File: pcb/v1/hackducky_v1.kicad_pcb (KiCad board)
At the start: 2 copper layers, 70 x 19 mm, 45 parts, among them J1 USB_C_Receptacle_USB2.0_16P, J2 Micro_SD_Card, J3 USB_A, SW1 SW_Push, SW2 SW_Push, U1 XC6206PxxxMR, U2 W25Q64JVZPIQ, U3 RP2040, Y1 Crystal_GND23

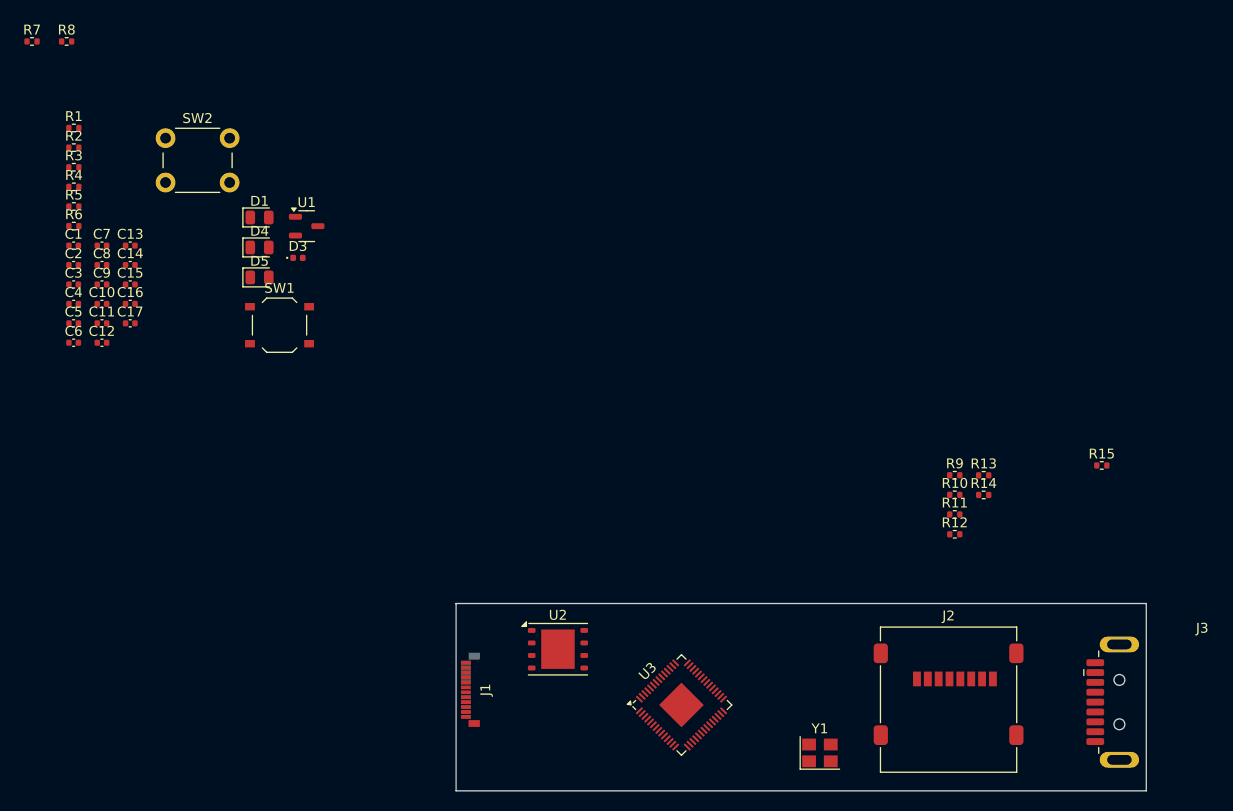
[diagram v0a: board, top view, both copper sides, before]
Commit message: edit stuff
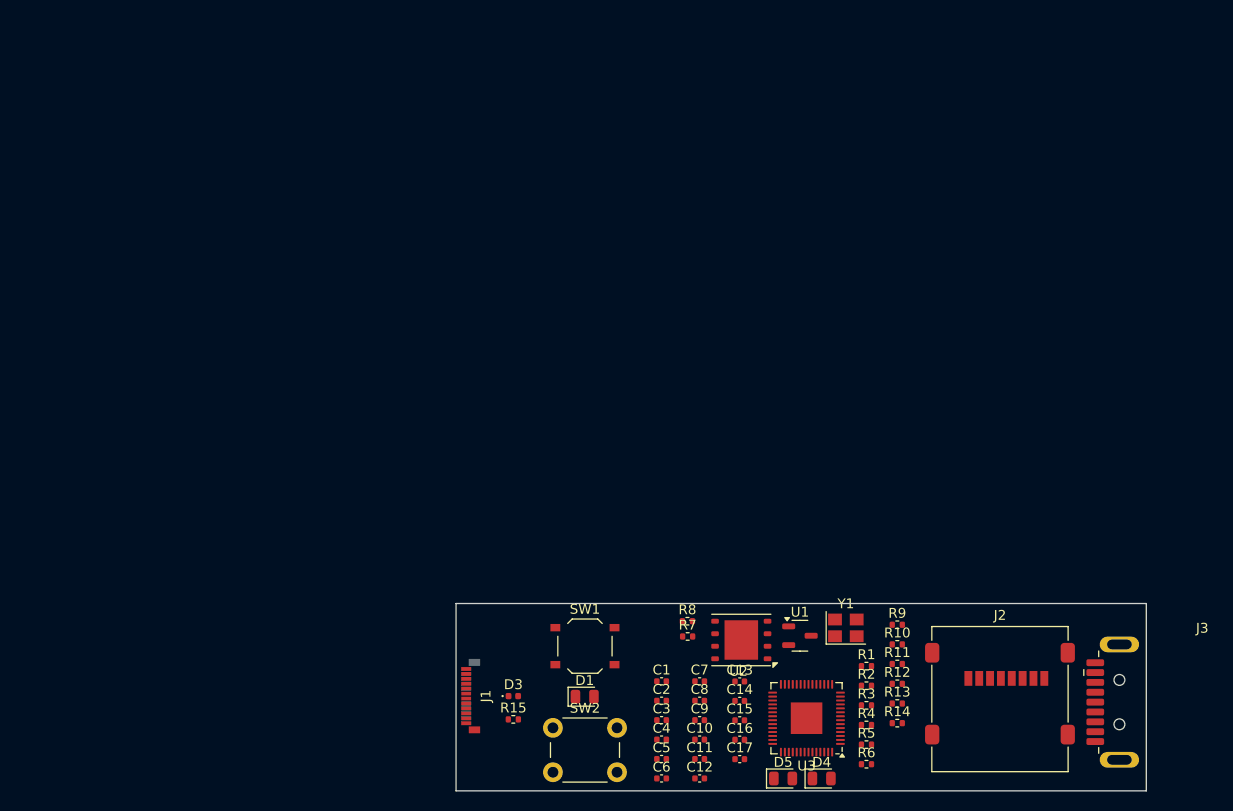
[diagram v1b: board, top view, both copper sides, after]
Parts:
- moved R1 97.2 mm to (120.6, 88.3)
- moved R2 97.2 mm to (120.6, 90.3)
- moved R3 97.2 mm to (120.6, 92.3)
- moved R4 97.2 mm to (120.6, 94.3)
- moved R5 97.2 mm to (120.6, 96.3)
- moved R6 97.2 mm to (120.6, 98.3)
- moved R7 89.8 mm to (102.5, 85.3)
- moved R8 86.1 mm to (102.5, 83.8)
- moved D4 78.4 mm to (116.1, 99.7)
- moved C15 76.0 mm to (107.8, 93.8)
- moved C16 76.0 mm to (107.8, 95.8)
- moved C17 76.0 mm to (107.8, 97.8)
- moved C13 76.0 mm to (107.8, 89.9)
- moved C14 76.0 mm to (107.8, 91.9)
- moved C7 75.0 mm to (103.7, 89.9)
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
